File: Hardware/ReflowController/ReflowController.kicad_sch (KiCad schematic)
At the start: 19 parts, among them J101 2060-1452, J102 2060-1452, J103 2060-1453, J104 2060-1452, J105 2060-1452, J106 2060-1452, J107 2060-1452, J108 2060-1452, J109 2060-1452, J110 2060-1452, J111 2060-1452, J112 2060-1452

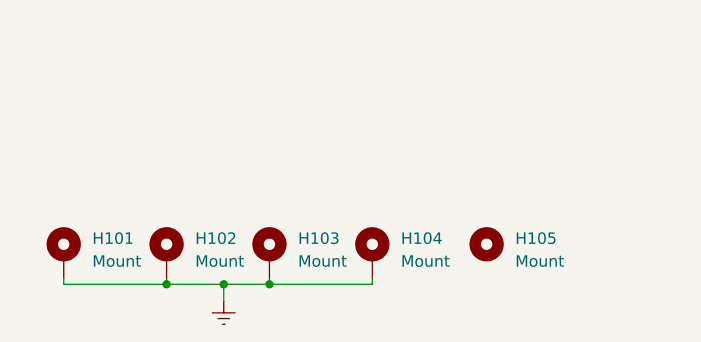
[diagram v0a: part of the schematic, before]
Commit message: working on DRC
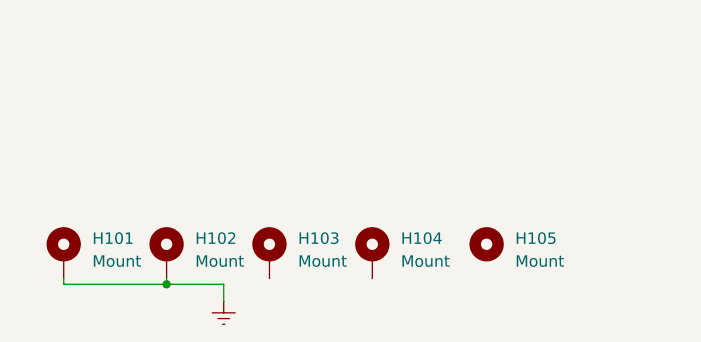
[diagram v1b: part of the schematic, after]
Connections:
- net Earth: no longer H103.1, H104.1
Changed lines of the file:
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@@
   (junction (at 190.5 21.59) (diameter 0) (color 0 0 0 0)
   )
-  (junction (at 35.56 189.865) (diameter 0) (color 0 0 0 0)
-  )
   (junction (at 36.195 131.445) (diameter 0) (color 0 0 0 0)
   )
   (junction (at 22.86 17.78) (diameter 0) (color 0 0 0 0)
   )
-  (junction (at 40.64 189.865) (diameter 0) (color 0 0 0 0)
-  )
   (junction (at 103.505 21.59) (diameter 0) (color 0 0 0 0)
   )
@@
     (stroke (width 0) (type default))
   )
-  (wire (pts (xy 40.64 189.23) (xy 40.64 189.865))
-    (stroke (width 0) (type default))
-  )
   (bus (pts (xy 209.55 109.855) (xy 209.55 112.395))
     (stroke (width 0) (type default))
@@
     (stroke (width 0) (type default))
   )
-  (wire (pts (xy 40.64 189.865) (xy 52.07 189.865))
-    (stroke (width 0) (type default))
-  )
   (wire (pts (xy 39.37 40.64) (xy 34.29 40.64))
     (stroke (width 0) (type default))
@@
     (stroke (width 0) (type default))
   )
-  (wire (pts (xy 52.07 189.865) (xy 52.07 189.23))
-    (stroke (width 0) (type default))
-  )
   (wire (pts (xy 212.09 80.645) (xy 228.6 80.645))
     (stroke (width 0) (type default))
@@
     (stroke (width 0) (type default))
   )
-  (wire (pts (xy 35.56 189.865) (xy 40.64 189.865))
-    (stroke (width 0) (type default))
-  )
